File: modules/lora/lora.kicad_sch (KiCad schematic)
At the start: 6 parts, among them U1 RFM95W-868S2

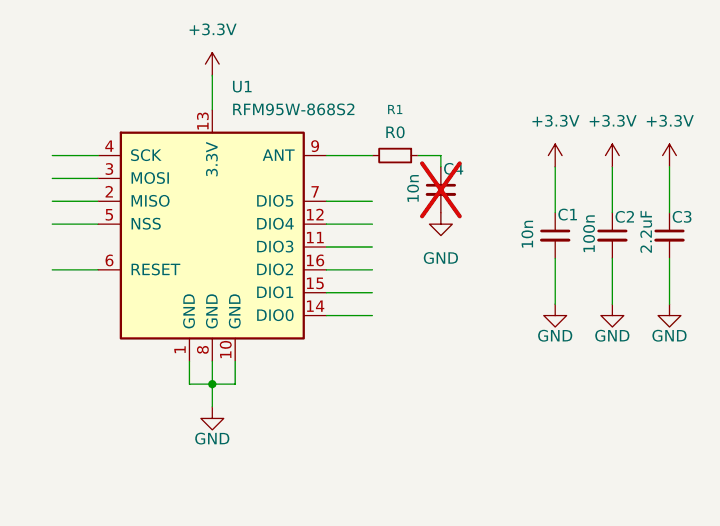
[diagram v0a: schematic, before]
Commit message: Updating all modules
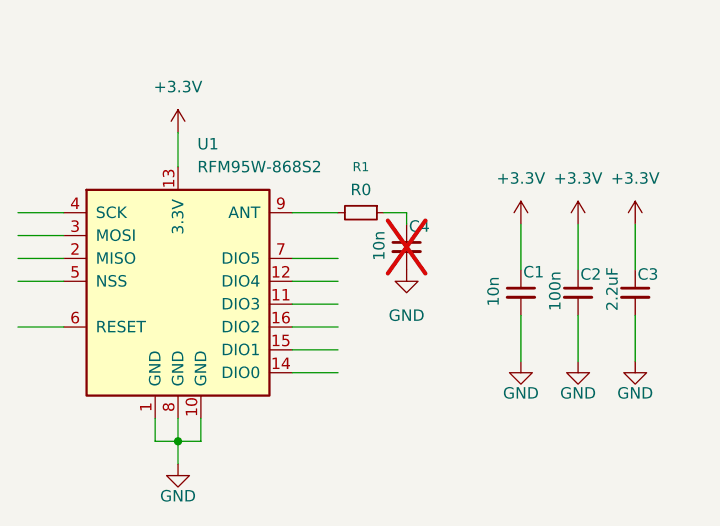
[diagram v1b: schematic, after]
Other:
- moved on the sheet: C1, C2, C3, C4, R1, U1

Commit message: Updating lora module
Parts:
- C1, C2, C3, C4: footprint (none) -> Capacitor_SMD:C_0603_1608Metric
- R1: footprint (none) -> Resistor_SMD:R_0603_1608Metric
- U1: footprint (none) -> RF_Module:HOPERF_RFM9XW_SMD
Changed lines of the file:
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@@
 			)
 		)
-		(property "Footprint" ""
+		(property "Footprint" "Capacitor_SMD:C_0603_1608Metric"
 			(at 120.65 62.23 0)
 			(effects
@@
 			)
 		)
-		(property "Footprint" ""
+		(property "Footprint" "Capacitor_SMD:C_0603_1608Metric"
 			(at 133.35 62.23 0)
 			(effects
@@
 			)
 		)
-		(property "Footprint" ""
+		(property "Footprint" "Resistor_SMD:R_0603_1608Metric"
 			(at 102.87 53.34 0)
 			(effects
@@
 			)
 		)
-		(property "Footprint" ""
+		(property "Footprint" "RF_Module:HOPERF_RFM9XW_SMD"
 			(at -1.27 19.05 0)
 			(effects
@@
 			)
 		)
-		(property "Footprint" ""
+		(property "Footprint" "Capacitor_SMD:C_0603_1608Metric"
 			(at 127 62.23 0)
 			(effects
@@
 			)
 		)
-		(property "Footprint" ""
+		(property "Footprint" "Capacitor_SMD:C_0603_1608Metric"
 			(at 107.95 57.15 0)
 			(effects
